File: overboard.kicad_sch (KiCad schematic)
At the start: 186 parts, among them J1 HRO-TYPE-C-31-M-12, J2 Conn_01x04, J3 Trackpoint, J4 Conn_01x04, J5 Conn_01x04, K00 Key_Switch, K01 Key_Switch, K02 Key_Switch, K03 Key_Switch, K10 Key_Switch, K11 Key_Switch, K12 Key_Switch, K13 Key_Switch, K20 Key_Switch, K21 Key_Switch, K22 Key_Switch, K23 Key_Switch, K30 Key_Switch, K31 Key_Switch, K32 Key_Switch, K33 Key_Switch, K40 Key_Switch, K41 Key_Switch, K42 Key_Switch, K43 Key_Switch, K50 Key_Switch, K51 Key_Switch, K52 Key_Switch, K53 Key_Switch, K92 Key_Switch, K93 Key_Switch, K94 Key_Switch, Q1 Q_NPN_Darlington_BCE, Q2 Q_NPN_Darlington_BCE, Q3 Q_NMOS_DGS, SW1 Reset_SW, U1 Teensy2.0++

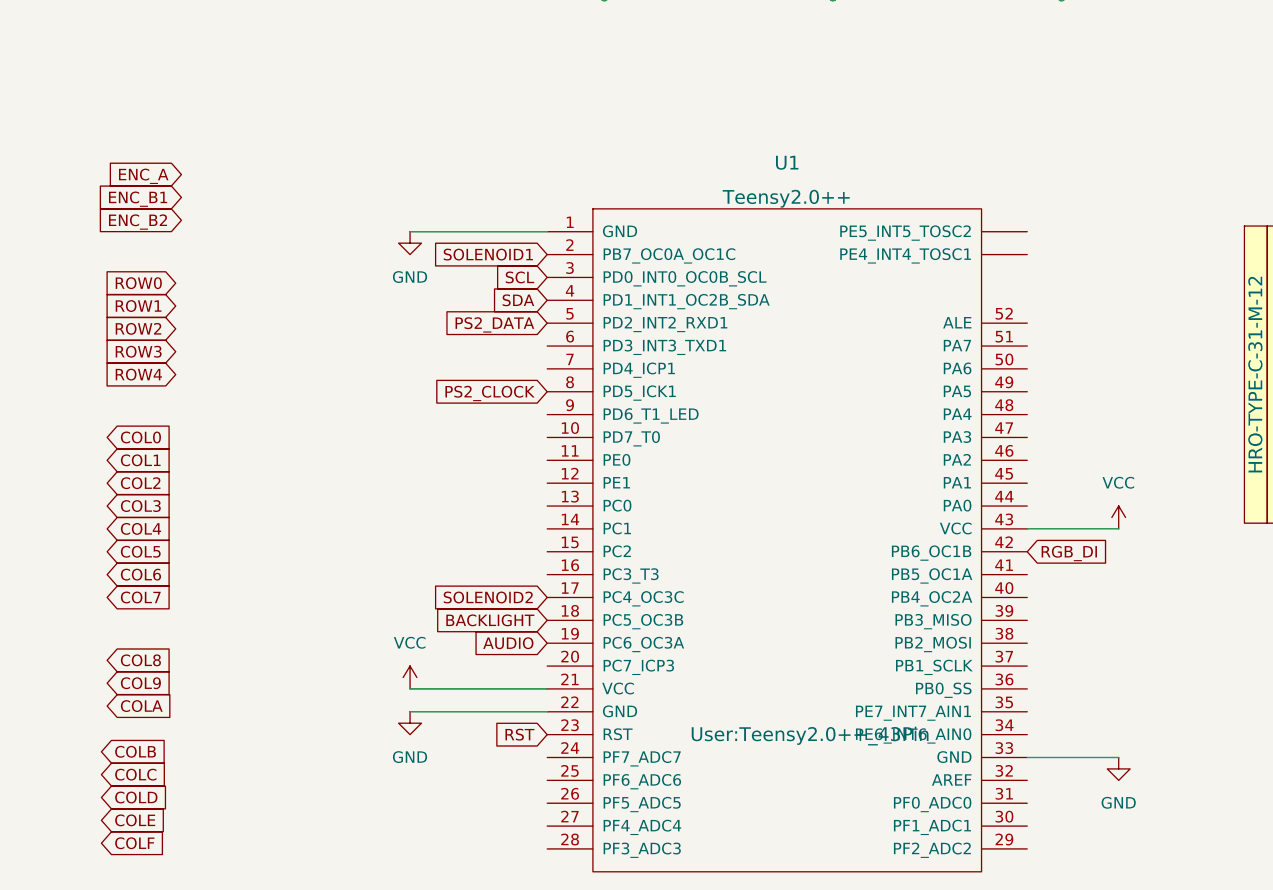
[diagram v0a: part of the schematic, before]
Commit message: Route PCB & plate
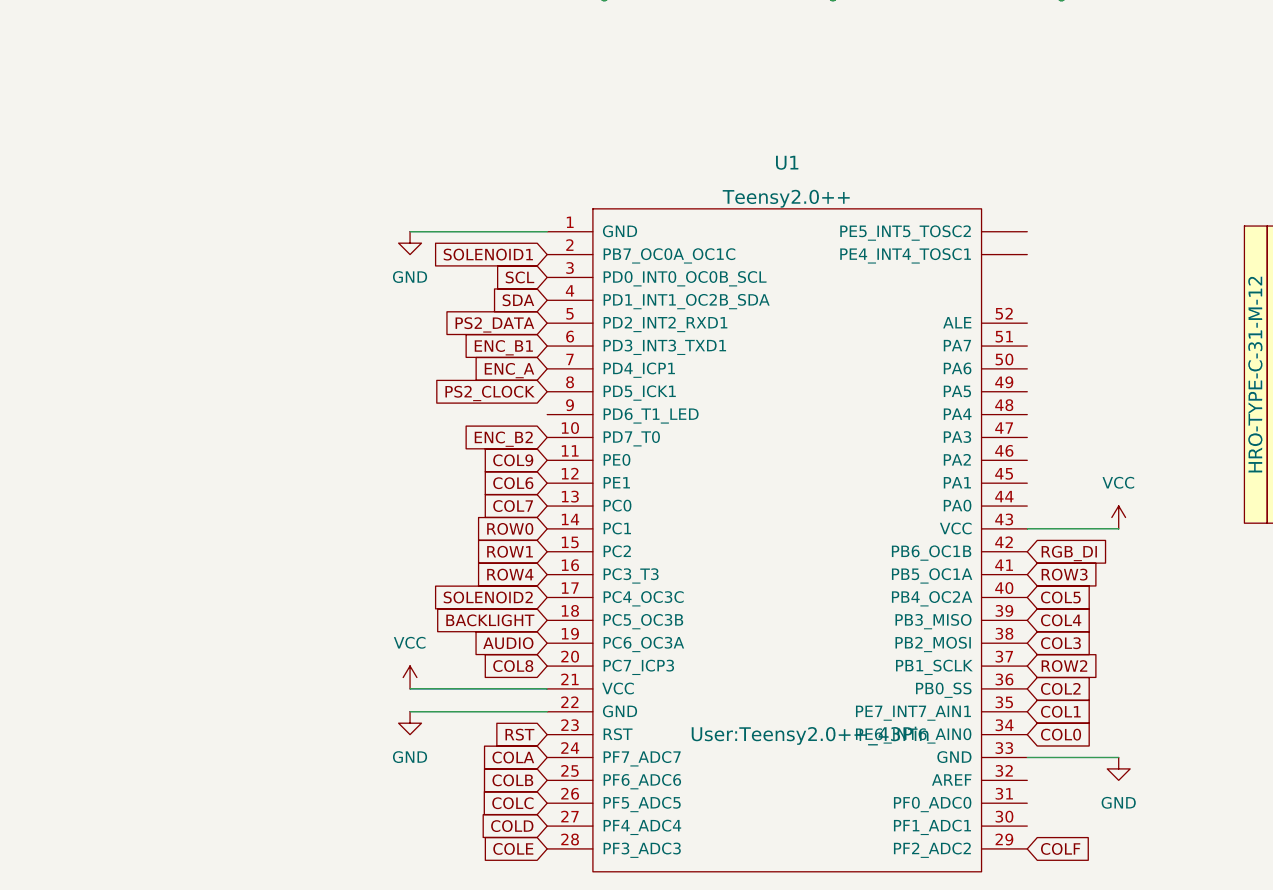
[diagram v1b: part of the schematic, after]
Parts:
- DL1, DL2: footprint Diode_THT:D_DO-41_SOD81_P7.62mm_Horizontal -> User:1N4001
- K00, K01, K02, K03, K10, K11, K12, K13, K20, K21, K22, K23, K30, K31, K32, K33, K40, K41, K42, K43, K50, K51, K52, K53, K92, K93, K94, KA0, KA1, KA2, KA3, KB0, KB1, KB2, KB3, KC0, KC1, KC2, KC3, KD0, KD1, KD2, KD3, KE0, KE1, KE2, KE3, KF0, KF1, KF2, KF3: footprint (none) -> User:MXOnly-1U
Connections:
- net COL0: now also U1.34 (PE6_INT6_AIN0)
- net COL1: now also U1.35 (PE7_INT7_AIN1)
- net COL2: now also U1.36 (PB0_SS)
- net COL3: now also U1.38 (PB2_MOSI)
- net COL4: now also U1.39 (PB3_MISO)
- net COL5: now also U1.40 (PB4_OC2A)
- net COL6: now also U1.12 (PE1)
- net COL7: now also U1.13 (PC0)
- net COL8: now also U1.20 (PC7_ICP3)
- net COL9: now also U1.11 (PE0)
- net COLA: now also U1.24 (PF7_ADC7)
- net COLB: now also U1.25 (PF6_ADC6)
- net COLC: now also U1.26 (PF5_ADC5)
- net COLD: now also U1.27 (PF4_ADC4)
- net COLE: now also U1.28 (PF3_ADC3)
- net COLF: now also U1.29 (PF2_ADC2)
- net ENC_A: now also U1.7 (PD4_ICP1)
- net ENC_B1: now also U1.6 (PD3_INT3_TXD1)
- net ENC_B2: now also U1.10 (PD7_T0)
- net ROW0: now also U1.14 (PC1)
- net ROW1: now also U1.15 (PC2)
- net ROW2: now also U1.37 (PB1_SCLK)
- net ROW3: now also U1.41 (PB5_OC1A)
- net ROW4: now also U1.16 (PC3_T3)
